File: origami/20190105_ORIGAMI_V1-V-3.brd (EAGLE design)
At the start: 32.7 x 12.1 mm, 5 parts, among them SW1 MK-12C02 G1.5, SW2 MK-12C02 G1.5

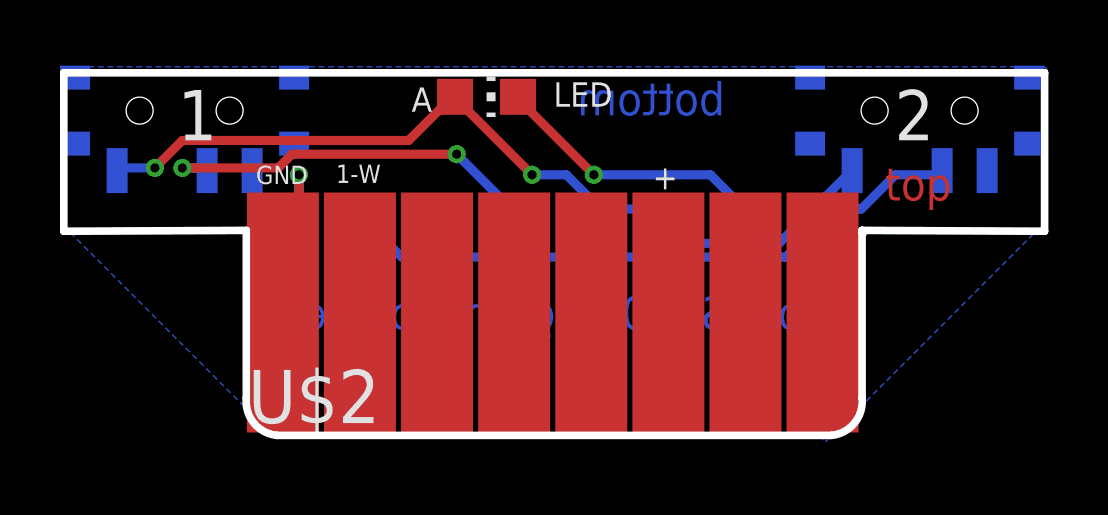
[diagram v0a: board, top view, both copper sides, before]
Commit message: fixed all and new switches
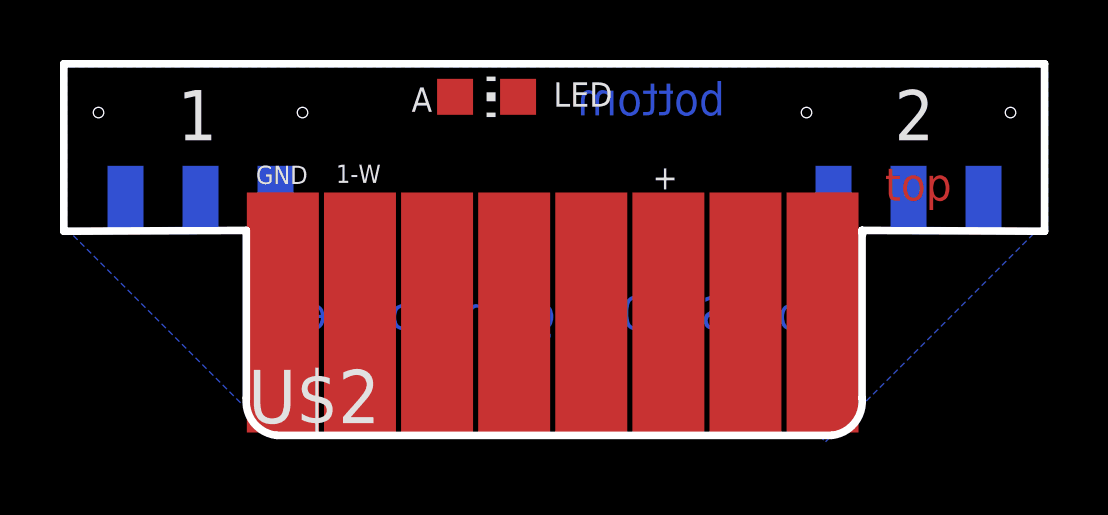
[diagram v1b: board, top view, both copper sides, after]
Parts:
- SW1, SW2: device SSSS810701:SSSS810701 -> _openSX70:K3-1280S-SMALL
- moved SW1 0.85 mm to (4.37, 12.8), turned to 0 degrees
- moved SW2 0.77 mm to (28.0, 12.8), turned to 0 degrees
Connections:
- net 2.8V-V: now also SW1.P$3, SW2.P$3; no longer SW1.1, SW2.1
- net N$2: now also SW2.P$2; no longer SW2.2
- net N$5: now also SW1.P$2; no longer SW1.2
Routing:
- net 2.8V-V: track 28.5 -> 0.00 mm, vias 2 -> 0
- net N$2: track 21.2 -> 0.00 mm
- net N$5: track 12.9 -> 0.00 mm, vias 2 -> 0
- net N$4: track 9.26 -> 0.00 mm, vias 1 -> 0
- net N$1: track 6.31 -> 0.00 mm, vias 1 -> 0
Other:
- board size 32.7 x 12.1 mm -> 32.7 x 12.4 mm
- board text added: "20190108_ORIGAMI_V3"
- board text removed: "20190108_ORIGAMI_V2"
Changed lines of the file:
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@@
 <text x="16.9312" y="13.0808" size="1.1" layer="16" font="vector" ratio="12" rot="MR180">bottom</text>
 <text x="25.3075" y="4.845" size="1.1" layer="16" font="vector" ratio="12" rot="MR0">openSX70 origami dongle</text>
-<text x="7.876" y="3.2764" size="1.016" layer="22" font="vector" rot="MR180">20190108_ORIGAMI_V2</text>
+<text x="7.876" y="3.2764" size="1.016" layer="22" font="vector" rot="MR180">20190108_ORIGAMI_V3</text>
 <text x="6.2131" y="9.693" size="0.6096" layer="25" font="vector">GND</text>
 <text x="8.8785" y="9.7295" size="0.6096" layer="25" font="vector">1-W</text>
@@
 <wire x1="5.892" y1="2.559" x2="5.892" y2="8.147" width="0.254" layer="20"/>
 <wire x1="5.892" y1="8.147" x2="-0.192" y2="8.119" width="0.254" layer="20"/>
-<wire x1="-0.192" y1="8.119" x2="-0.192" y2="13.4" width="0.254" layer="20"/>
-<wire x1="-0.192" y1="13.4" x2="32.5" y2="13.4" width="0.254" layer="20"/>
-<wire x1="32.5" y1="13.4" x2="32.5" y2="8.119" width="0.254" layer="20"/>
+<wire x1="-0.192" y1="8.119" x2="-0.192" y2="13.7" width="0.254" layer="20"/>
+<wire x1="-0.192" y1="13.7" x2="32.5" y2="13.7" width="0.254" layer="20"/>
+<wire x1="32.5" y1="13.7" x2="32.5" y2="8.119" width="0.254" layer="20"/>
 <wire x1="32.5" y1="8.119" x2="26.416" y2="8.147" width="0.254" layer="20"/>
 <wire x1="26.416" y1="8.147" x2="26.438" y2="8.02" width="0.254" layer="20"/>
@@
 </autorouter>
 <elements>
-<element name="SW1" library="SSSS810701" package="SSSS810701" value="MK-12C02 G1.5" x="3.835" y="12.14" rot="MR180">
-<attribute name="AVAILABILITY" value="Good" x="3.835" y="12.14" size="1.778" layer="28" rot="MR180" display="off"/>
-<attribute name="DESCRIPTION" value=" Slide Switch • Rating (max.): 0.3 A 5 VDC • Poles: 1 • Positions: 2 • Travel : 1.5 mm • Operating direction: Horizontal " x="3.835" y="12.14" size="1.778" layer="28" rot="MR180" display="off"/>
-<attribute name="MF" value="ALPS" x="3.835" y="12.14" size="1.778" layer="28" rot="MR180" display="off"/>
-<attribute name="MP" value="SSSS810701" x="3.835" y="12.14" size="1.778" layer="28" rot="MR180" display="off"/>
-<attribute name="PACKAGE" value="None" x="3.835" y="12.14" size="1.778" layer="28" rot="MR180" display="off"/>
-<attribute name="PRICE" value="0.53 USD" x="3.835" y="12.14" size="1.778" layer="28" rot="MR180" display="off"/>
-</element>
-<element name="SW2" library="SSSS810701" package="SSSS810701" value="MK-12C02 G1.5" x="28.335" y="12.14" rot="MR180">
-<attribute name="AVAILABILITY" value="Good" x="28.335" y="12.14" size="1.778" layer="28" rot="MR180" display="off"/>
-<attribute name="DESCRIPTION" value=" Slide Switch • Rating (max.): 0.3 A 5 VDC • Poles: 1 • Positions: 2 • Travel : 1.5 mm • Operating direction: Horizontal " x="28.335" y="12.14" size="1.778" layer="28" rot="MR180" display="off"/>
-<attribute name="MF" value="ALPS" x="28.335" y="12.14" size="1.778" layer="28" rot="MR180" display="off"/>
-<attribute name="MP" value="SSSS810701" x="28.335" y="12.14" size="1.778" layer="28" rot="MR180" display="off"/>
-<attribute name="PACKAGE" value="None" x="28.335" y="12.14" size="1.778" layer="28" rot="MR180" display="off"/>
-<attribute name="PRICE" value="0.53 USD" x="28.335" y="12.14" size="1.778" layer="28" rot="MR180" display="off"/>
-</element>
+<element name="SW1" library="_openSX70" library_urn="urn:adsk.eagle:library:7902803" package="K3-1280S-SMALL" value="MK-12C02 G1.5" x="4.365" y="12.81" rot="MR0"/>
+<element name="SW2" library="_openSX70" library_urn="urn:adsk.eagle:library:7902803" package="K3-1280S-SMALL" value="MK-12C02 G1.5" x="27.965" y="12.81" rot="MR0"/>
 <element name="U$1" library="_openSX70" library_urn="urn:adsk.eagle:library:7902803" package="FLASH-8-BRIDGE-SW1-SW2-LED-SMALL" package3d_urn="urn:adsk.eagle:package:7902950/1" value="FLASH-BRIDGE-SW1-SW2-LED-SMALL" x="16.1" y="13.7" rot="MR180"/>
 <element name="U$2" library="_openSX70" library_urn="urn:adsk.eagle:library:7902803" package="SX70-FLASH-EDGE8-2" package3d_urn="urn:adsk.eagle:package:7902946/1" value="SX70-FLASH-EDGE8-MALE-LONG" x="16.11" y="-2.089"/>
@@
 <contactref element="U$1" pad="VCC-2.8V"/>
 <contactref element="LED" pad="A"/>
-<contactref element="SW2" pad="1"/>
-<contactref element="SW1" pad="1"/>
-<wire x1="15.4174" y1="10.0012" x2="12.9028" y2="12.5158" width="0.3048" layer="1"/>
-<wire x1="16.5604" y1="10.0012" x2="15.4174" y2="10.0012" width="0.3048" layer="16"/>
-<wire x1="17.7034" y1="8.8582" x2="16.5604" y2="10.0012" width="0.3048" layer="16"/>
-<wire x1="19.7608" y1="8.8582" x2="17.7034" y2="8.8582" width="0.3048" layer="16"/>
-<wire x1="12.9028" y1="12.5158" x2="12.85" y2="12.6" width="0.3048" layer="1"/>
-<wire x1="19.95" y1="8.74" x2="19.7608" y2="8.8582" width="0.3048" layer="16"/>
-<wire x1="2.8444" y1="10.2298" x2="1.7014" y2="10.2298" width="0.3048" layer="16"/>
-<wire x1="3.7588" y1="11.1442" x2="2.8444" y2="10.2298" width="0.3048" layer="1"/>
-<wire x1="11.3026" y1="11.1442" x2="3.7588" y2="11.1442" width="0.3048" layer="1"/>
-<wire x1="12.6742" y1="12.5158" x2="11.3026" y2="11.1442" width="0.3048" layer="1"/>
-<wire x1="1.7014" y1="10.2298" x2="1.585" y2="10.14" width="0.3048" layer="16"/>
-<wire x1="12.85" y1="12.6" x2="12.6742" y2="12.5158" width="0.3048" layer="1"/>
-<wire x1="25.933" y1="10.0012" x2="23.647" y2="7.7152" width="0.3048" layer="16"/>
-<wire x1="23.647" y1="7.7152" x2="20.9038" y2="7.7152" width="0.3048" layer="16"/>
-<wire x1="20.9038" y1="7.7152" x2="19.9894" y2="8.6296" width="0.3048" layer="16"/>
-<wire x1="26.085" y1="10.14" x2="25.933" y2="10.0012" width="0.3048" layer="16"/>
-<wire x1="19.9894" y1="8.6296" x2="19.95" y2="8.74" width="0.3048" layer="16"/>
-<via x="15.4174" y="10.0012" extent="1-16" drill="0.3048"/>
-<via x="2.8444" y="10.2298" extent="1-16" drill="0.3048"/>
+<contactref element="SW2" pad="P$3"/>
+<contactref element="SW1" pad="P$3"/>
+<wire x1="19.95" y1="8.74" x2="25.465" y2="9.2" width="0" layer="19" extent="16-16"/>
+<wire x1="12.85" y1="12.6" x2="19.95" y2="8.74" width="0" layer="19" extent="1-16"/>
+<wire x1="1.865" y1="9.2" x2="12.85" y2="12.6" width="0" layer="19" extent="1-16"/>
 </signal>
 <signal name="N$1">
 <contactref element="U$2" pad="GND"/>
 <contactref element="U$1" pad="GND"/>
-<wire x1="7.645" y1="10.0012" x2="7.645" y2="8.6296" width="0.3048" layer="16"/>
-<wire x1="7.645" y1="10.0012" x2="7.645" y2="5.8864" width="0.3048" layer="1"/>
-<wire x1="7.645" y1="5.8864" x2="7.1878" y2="5.4292" width="0.3048" layer="1"/>
-<wire x1="7.7096" y1="8.5622" x2="7.645" y2="8.6296" width="0.3048" layer="16"/>
-<wire x1="7.1878" y1="5.4292" x2="7.11" y2="5.411" width="0.3048" layer="1"/>
-<via x="7.645" y="10.0012" extent="1-16" drill="0.3048"/>
+<wire x1="7.11" y1="5.411" x2="7.7096" y2="8.5622" width="0" layer="19" extent="1-16"/>
 </signal>
 <signal name="N$4">
 <contactref element="U$1" pad="LED"/>
 <contactref element="LED" pad="C"/>
-<wire x1="17.4748" y1="10.0012" x2="14.9602" y2="12.5158" width="0.3048" layer="1"/>
-<wire x1="21.361" y1="10.0012" x2="17.4748" y2="10.0012" width="0.3048" layer="16"/>
-<wire x1="22.504" y1="8.8582" x2="21.361" y2="10.0012" width="0.3048" layer="16"/>
-<wire x1="14.9602" y1="12.5158" x2="14.95" y2="12.6" width="0.3048" layer="1"/>
-<wire x1="22.52" y1="8.74" x2="22.504" y2="8.8582" width="0.3048" layer="16"/>
-<via x="17.4748" y="10.0012" extent="1-16" drill="0.3048"/>
+<wire x1="14.95" y1="12.6" x2="22.52" y2="8.74" width="0" layer="19" extent="1-16"/>
 </signal>
 <signal name="GND">
 <polygon width="0.1524" layer="16">
-<vertex x="-0.2" y="13.5"/>
-<vertex x="-0.2" y="8.3"/>
+<vertex x="-0.1" y="13.6"/>
+<vertex x="-0.1" y="8.2"/>
 <vertex x="6.8" y="1.3"/>
 <vertex x="25" y="1.3"/>
@@
 <vertex x="32.6" y="13.5"/>
 <vertex x="32.5" y="13.6"/>
-<vertex x="-0.1" y="13.6"/>
 </polygon>
 </signal>
 <signal name="N$2">
-<contactref element="SW2" pad="2"/>
+<contactref element="SW2" pad="P$2"/>
 <contactref element="U$1" pad="SWITCH-2"/>
-<wire x1="28.9048" y1="10.0012" x2="27.5332" y2="10.0012" width="0.3048" layer="16"/>
-<wire x1="27.5332" y1="10.0012" x2="26.3902" y2="8.8582" width="0.3048" layer="16"/>
-<wire x1="26.3902" y1="8.8582" x2="25.4758" y2="8.8582" width="0.3048" layer="16"/>
-<wire x1="25.4758" y1="8.8582" x2="23.8756" y2="7.258" width="0.3048" layer="16"/>
-<wire x1="23.8756" y1="7.258" x2="11.074" y2="7.258" width="0.3048" layer="16"/>
-<wire x1="11.074" y1="7.258" x2="9.7024" y2="8.6296" width="0.3048" layer="16"/>
-<wire x1="29.085" y1="10.14" x2="28.9048" y2="10.0012" width="0.3048" layer="16"/>
-<wire x1="9.7024" y1="8.6296" x2="9.67" y2="8.74" width="0.3048" layer="16"/>
+<wire x1="9.67" y1="8.74" x2="27.965" y2="9.2" width="0" layer="19" extent="16-16"/>
 </signal>
 <signal name="N$5">
-<contactref element="SW1" pad="2"/>
+<contactref element="SW1" pad="P$2"/>
 <contactref element="U$1" pad="SWITCH-1"/>
-<wire x1="4.4446" y1="10.2298" x2="3.7588" y2="10.2298" width="0.3048" layer="16"/>
-<wire x1="6.9592" y1="10.2298" x2="3.7588" y2="10.2298" width="0.3048" layer="1"/>
-<wire x1="7.4164" y1="10.687" x2="6.9592" y2="10.2298" width="0.3048" layer="1"/>
-<wire x1="12.9028" y1="10.687" x2="7.4164" y2="10.687" width="0.3048" layer="1"/>
-<wire x1="14.7316" y1="8.8582" x2="12.9028" y2="10.687" width="0.3048" layer="16"/>
-<wire x1="4.585" y1="10.14" x2="4.4446" y2="10.2298" width="0.3048" layer="16"/>
-<wire x1="14.81" y1="8.74" x2="14.7316" y2="8.8582" width="0.3048" layer="16"/>
-<via x="3.7588" y="10.2298" extent="1-16" drill="0.3048"/>
-<via x="12.9028" y="10.687" extent="1-16" drill="0.3048"/>
+<wire x1="4.365" y1="9.2" x2="14.81" y2="8.74" width="0" layer="19" extent="16-16"/>
 </signal>
 </signals>
